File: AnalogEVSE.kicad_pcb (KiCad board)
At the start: 2 copper layers, 102.3 x 84.5 mm, 79 parts, among them K1 Relay, P1 Pilot, P2 Rext, P3 230V, P4 Relay 1, P5 Status LEDs, P6 Power, P7 Relay 2, Q1 BC337-40, Q2 BC337-40, Q3 BC557, Q4 BC337-40, T1 12V/3VA, U1 LM2901, U2 LM7812, U3 LM7912, U4 LM2901

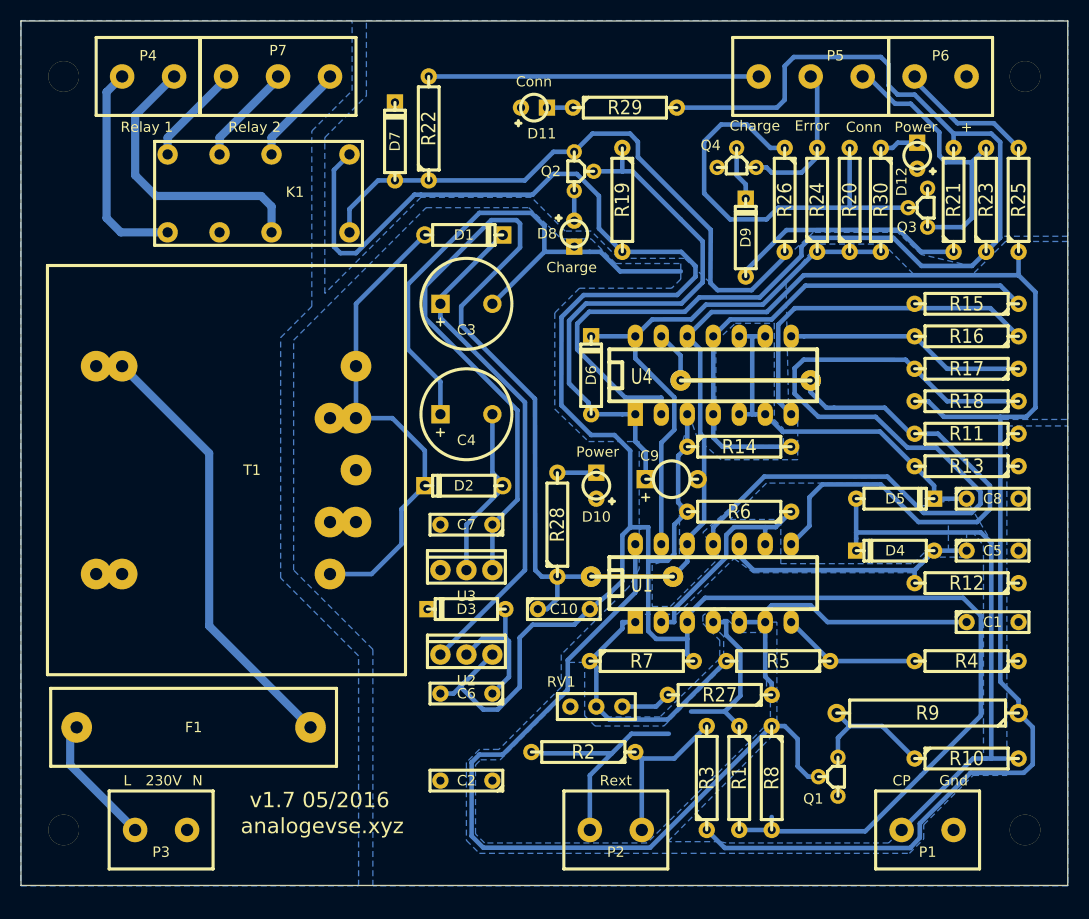
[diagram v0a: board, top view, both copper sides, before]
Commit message: RV2
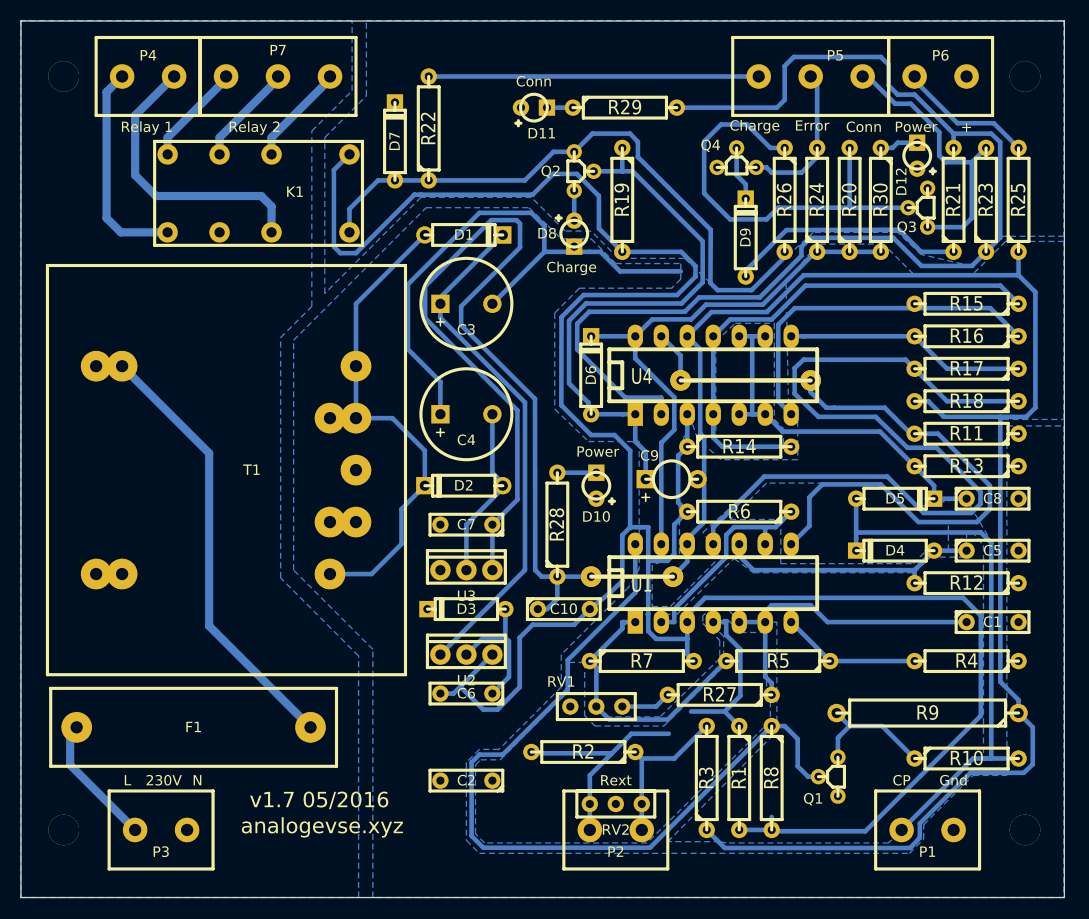
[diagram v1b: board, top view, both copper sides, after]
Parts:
- added RV2: 10k, mylib:Trimpot, F.Cu at (99.1, 109.9)
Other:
- board size 102.3 x 84.5 mm -> 102 x 85.7 mm
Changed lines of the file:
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@@
 (kicad_pcb (version 4) (host pcbnew no-vcs-found-product)
   (general
-    (links 145)
+    (links 148)
     (no_connects 0)
-    (area 40.859999 33.259999 143.290001 117.870001)
+    (area 39.303667 32.139 145.100334 119.050001)
     (thickness 1.6)
     (drawings 28)
-    (tracks 479)
+    (tracks 480)
     (zones 0)
-    (modules 79)
+    (modules 80)
     (nets 50)
   )
@@
       (net 25 "Net-(K1-Pad16)"))
   )
+  (module mylib:Trimpot placed (layer F.Cu)
+    (at 99.06 109.855)
+    (fp_text reference RV2 (at 0 2.54) (layer F.SilkS)
+      (effects (font (size 1.016 1.016) (thickness 0.2032)))
+    )
+    (fp_text value 10k (at 0 -2.54) (layer F.SilkS) hide
+      (effects (font (size 1.016 1.016) (thickness 0.2032)))
+    )
+    (fp_line (start -3.81 -1.27) (end -3.81 1.27) (layer F.SilkS) (width 0.3048))
+    (fp_line (start -3.81 1.27) (end 3.81 1.27) (layer F.SilkS) (width 0.3048))
+    (fp_line (start 3.81 1.27) (end 3.81 -1.27) (layer F.SilkS) (width 0.3048))
+    (fp_line (start 3.81 -1.27) (end -3.81 -1.27) (layer F.SilkS) (width 0.3048))
+    (pad 1 thru_hole circle (at -2.54 0) (size 1.6 1.6) (drill 0.8) (layers *.Cu *.Mask F.SilkS)
+      (net 9 "Net-(C2-Pad1)"))
+    (pad 2 thru_hole circle (at 0 0) (size 1.6 1.6) (drill 0.8) (layers *.Cu *.Mask F.SilkS)
+      (net 9 "Net-(C2-Pad1)"))
+    (pad 3 thru_hole circle (at 2.54 0) (size 1.6 1.6) (drill 0.8) (layers *.Cu *.Mask F.SilkS)
+      (net 31 "Net-(P2-Pad2)"))
+  )
   (gr_text Charge (at 94.742 57.404) (layer F.SilkS)
     (effects (font (size 1 1) (thickness 0.2)))
@@
     (effects (font (size 1.5 1.5) (thickness 0.3)))
   )
-  (gr_line (start 40.91 117.82) (end 40.91 33.31) (angle 90) (layer Edge.Cuts) (width 0.1))
-  (gr_line (start 143.24 117.82) (end 40.91 117.82) (angle 90) (layer Edge.Cuts) (width 0.1))
-  (gr_line (start 143.24 33.31) (end 143.24 117.82) (angle 90) (layer Edge.Cuts) (width 0.1))
-  (gr_line (start 40.91 33.31) (end 143.24 33.31) (angle 90) (layer Edge.Cuts) (width 0.1))
+  (gr_line (start 40.91 119) (end 40.91 33.31) (angle 90) (layer Edge.Cuts) (width 0.1))
+  (gr_line (start 142.91 119) (end 40.91 119) (angle 90) (layer Edge.Cuts) (width 0.1))
+  (gr_line (start 142.91 33.31) (end 142.91 119) (angle 90) (layer Edge.Cuts) (width 0.1))
+  (gr_line (start 40.91 33.31) (end 142.91 33.31) (angle 90) (layer Edge.Cuts) (width 0.1))
   (segment (start 100.463 82.81) (end 100.463 75.317) (width 0.45) (layer B.Cu) (net 1))
   (segment (start 100.463 75.317) (end 98.933 73.787) (width 0.45) (layer B.Cu) (net 1))
@@
   (segment (start 66.04 38.989) (end 66.04 38.735) (width 0.8) (layer B.Cu) (net 30))
   (segment (start 100.965 104.775) (end 101.6 105.41) (width 0.45) (layer B.Cu) (net 31))
-  (segment (start 101.6 105.41) (end 101.6 112.395) (width 0.45) (layer B.Cu) (net 31))
+  (segment (start 101.6 105.41) (end 101.6 109.855) (width 0.45) (layer B.Cu) (net 31))
+  (segment (start 101.6 109.855) (end 101.6 112.395) (width 0.45) (layer B.Cu) (net 31))
   (segment (start 104.775 105.41) (end 107.95 102.235) (width 0.45) (layer B.Cu) (net 31))
   (segment (start 101.6 105.41) (end 104.775 105.41) (width 0.45) (layer B.Cu) (net 31))
@@
     (polygon
       (pts
-        (xy 143.256 54.356) (xy 136.652 54.356) (xy 133.858 57.277) (xy 128.905 56.134) (xy 126.619 53.975)
+        (xy 142.875 54.356) (xy 136.652 54.356) (xy 133.858 57.277) (xy 128.905 56.134) (xy 126.619 53.975)
         (xy 118.364 53.975) (xy 112.268 59.563) (xy 108.966 59.563) (xy 105.791 56.515) (xy 99.314 56.515)
         (xy 96.647 53.848) (xy 94.107 53.848) (xy 90.805 50.546) (xy 80.01 50.546) (xy 70.612 59.944)
-        (xy 70.612 44.704) (xy 74.676 40.64) (xy 74.676 33.274) (xy 143.256 33.274)
+        (xy 70.612 44.704) (xy 74.676 40.64) (xy 74.676 33.274) (xy 142.875 33.274)
       )
     )
@@
         (xy 93.726 98.425) (xy 87.63 104.521) (xy 85.725 104.521) (xy 84.455 105.791) (xy 84.455 113.411)
         (xy 85.725 114.681) (xy 127.762 114.681) (xy 129.159 113.284) (xy 129.159 111.887) (xy 133.985 107.061)
-        (xy 137.287 107.061) (xy 137.287 72.898) (xy 143.256 72.898) (xy 143.256 117.856) (xy 75.311 117.856)
+        (xy 137.287 107.061) (xy 137.287 72.898) (xy 142.875 72.898) (xy 142.875 118.999) (xy 75.311 118.999)
         (xy 75.311 94.742) (xy 67.564 86.995) (xy 67.564 64.516) (xy 80.518 51.562) (xy 90.551 51.562)
         (xy 92.456 53.34) (xy 93.726 54.61) (xy 96.647 54.61) (xy 99.06 57.023) (xy 105.41 57.023)
@@
     (polygon
       (pts
-        (xy 143.256 54.864) (xy 137.16 54.864) (xy 133.985 58.039) (xy 128.143 58.039) (xy 125.222 55.118)
+        (xy 142.875 54.864) (xy 137.16 54.864) (xy 133.985 58.039) (xy 128.143 58.039) (xy 125.222 55.118)
         (xy 118.745 55.118) (xy 115.697 58.928) (xy 115.951 71.247) (xy 116.84 72.39) (xy 116.84 76.2)
         (xy 109.347 76.2) (xy 107.061 74.168) (xy 106.299 72.009) (xy 105.156 75.946) (xy 105.283 82.042)
         (xy 105.283 85.598) (xy 102.616 86.487) (xy 102.616 90.551) (xy 104.394 90.551) (xy 109.22 85.725)
         (xy 107.569 83.312) (xy 113.665 77.851) (xy 125.603 77.978) (xy 128.778 80.772) (xy 133.223 79.883)
-        (xy 136.652 85.725) (xy 136.652 72.136) (xy 136.906 72.263) (xy 138.811 72.263) (xy 143.256 72.263)
+        (xy 136.652 85.725) (xy 136.652 72.136) (xy 136.906 72.263) (xy 138.811 72.263) (xy 142.875 72.263)
       )
     )
@@
     (polygon
       (pts
-        (xy 40.894 33.274) (xy 40.894 117.856) (xy 73.914 117.856) (xy 73.914 95.377) (xy 66.294 87.757)
+        (xy 40.894 33.274) (xy 40.894 118.999) (xy 73.914 118.999) (xy 73.914 95.377) (xy 66.294 87.757)
         (xy 66.294 64.262) (xy 69.342 61.214) (xy 69.342 44.069) (xy 73.279 40.132) (xy 73.279 33.274)
       )
